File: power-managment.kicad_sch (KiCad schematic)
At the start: 9 parts, among them U1 MPM3610GQV-P

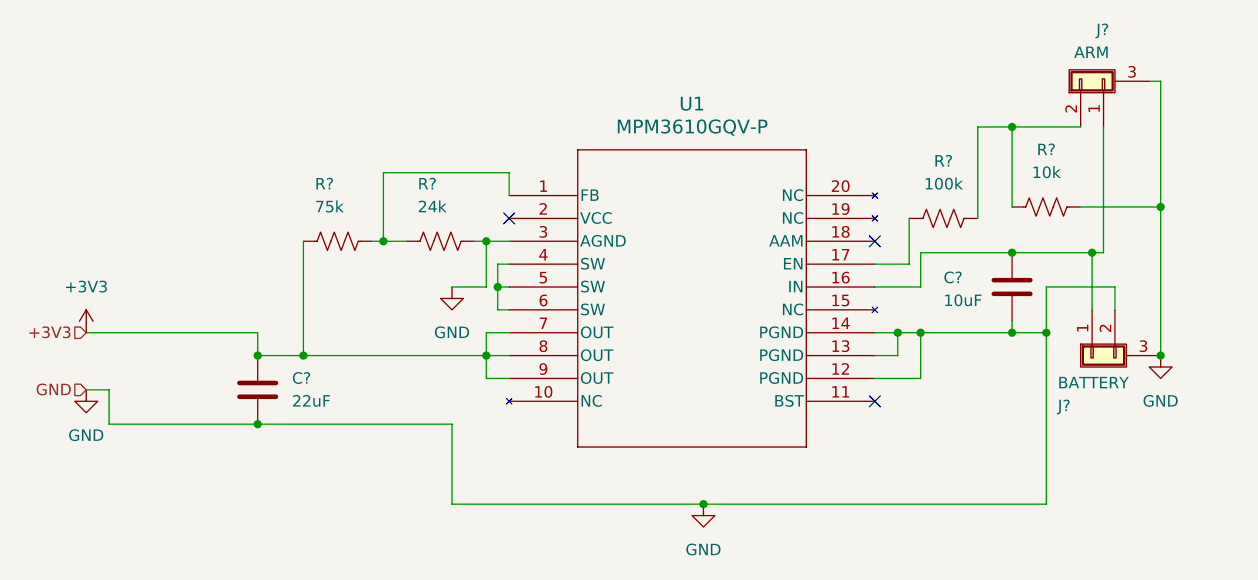
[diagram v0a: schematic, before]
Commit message: Julia cleaning wires
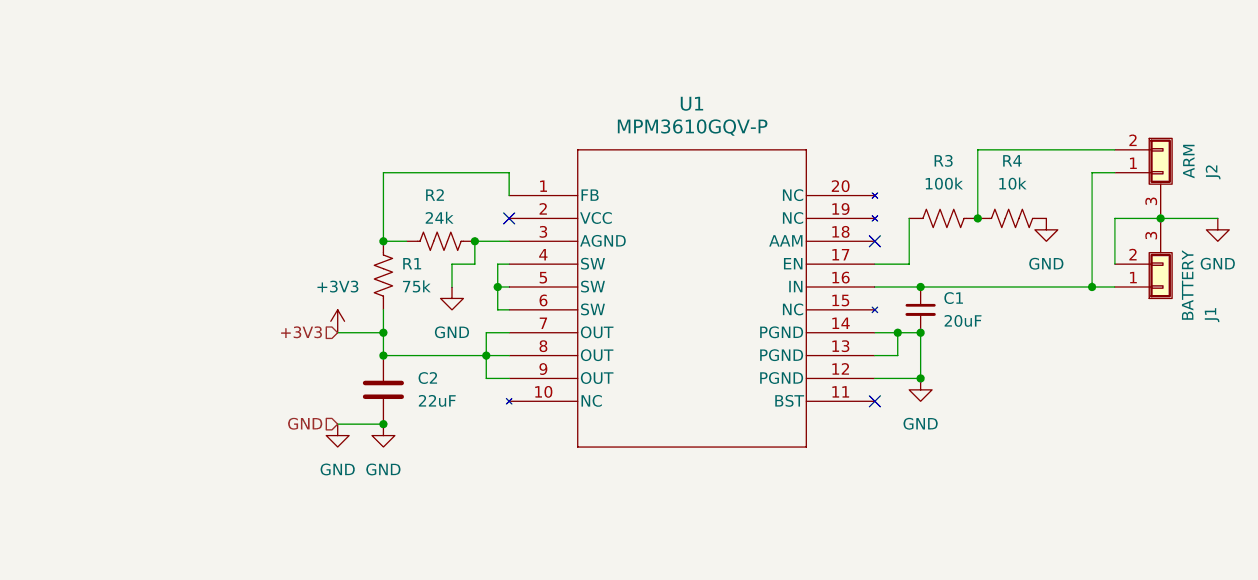
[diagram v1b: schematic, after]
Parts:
- removed C?: 10uF, symbol Device:C
- removed J?: BATTERY, Avionics_Feet:0436500205, symbol Connector_Generic_Shielded:Conn_01x02_Shielded
- added C1: 20uF, symbol Device:C_Small
- added J1: BATTERY, Avionics_Feet:0436500205, symbol Connector_Generic_Shielded:Conn_01x02_Shielded
- gave numbers to parts that had none: 6
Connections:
- net GND: now also C1.2, J1.2 (Pin_2), J1.3 (Shield)
- net at J2.1 (Pin_2), U1.16 (IN): now also C1.1, J1.1 (Pin_1)
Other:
- moved on the sheet: C2, J2, R1, R4
